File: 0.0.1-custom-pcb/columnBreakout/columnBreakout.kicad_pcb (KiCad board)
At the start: 2 copper layers, 14.7 x 63.3 mm, 7 parts, among them J1 HC-FPC-0.5-12P-FH20, J2 HC-FPC-0.5-6P-FH20, J3 HC-FPC-0.5-6P-FH20, J4 HC-FPC-0.5-6P-FH20, J5 HC-FPC-0.5-6P-FH20, J6 HC-FPC-0.5-6P-FH20, J7 HC-FPC-0.5-6P-FH20

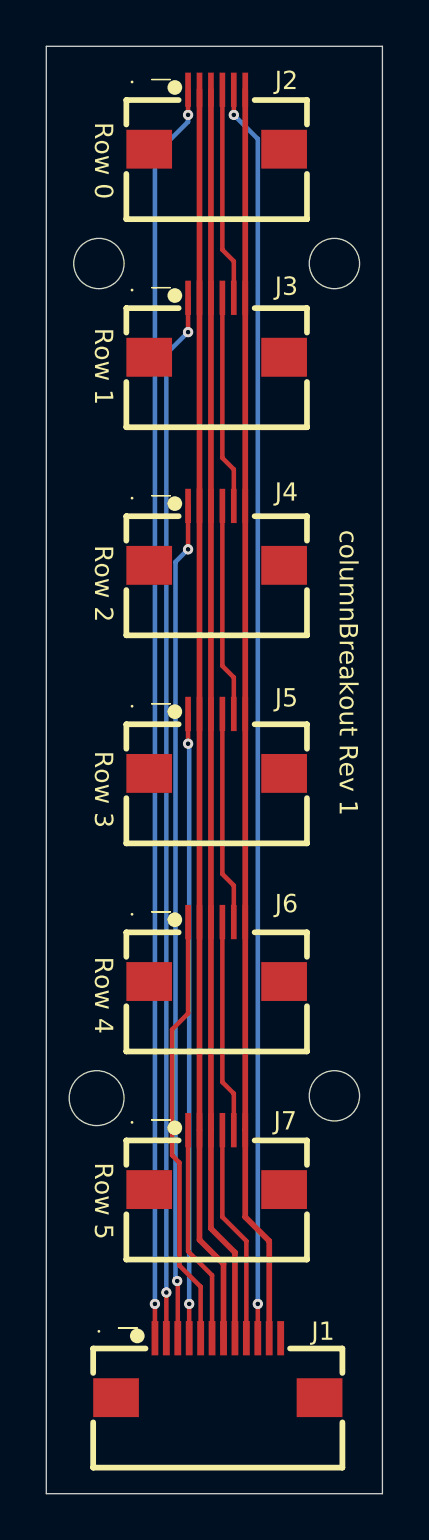
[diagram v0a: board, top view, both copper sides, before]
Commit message: final changes to columnBreakout
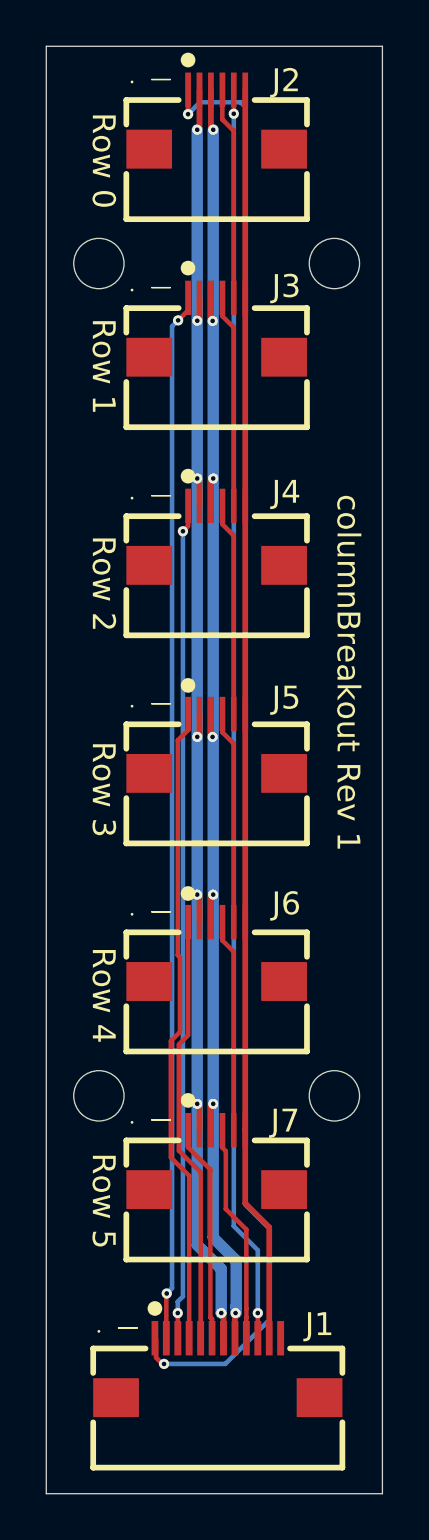
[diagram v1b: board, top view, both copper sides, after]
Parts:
- added H1: MountingHole_2.2mm_M2_4.4mmHead, Mechanical:MountingHole_2.2mm_M2_4.4mmHead, F.Cu at (148.8, 51.5)
- added H2: MountingHole_2.2mm_M2_4.4mmHead, Mechanical:MountingHole_2.2mm_M2_4.4mmHead, F.Cu at (159.1, 51.5)
- added H3: MountingHole_2.2mm_M2_4.4mmHead, Mechanical:MountingHole_2.2mm_M2_4.4mmHead, F.Cu at (148.8, 87.9)
- added H4: MountingHole_2.2mm_M2_4.4mmHead, Mechanical:MountingHole_2.2mm_M2_4.4mmHead, F.Cu at (159.1, 87.9)
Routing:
- net /R0: track 55.2 -> 64.1 mm
- net /VDD: track 55.0 -> 61.1 mm, vias 0 -> 7
- net /GND: track 55.0 -> 60.9 mm, vias 0 -> 7
- net /R3: track 27.3 -> 28.0 mm, vias 2 -> 0
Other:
- outline, holes or cut-outs redrawn
